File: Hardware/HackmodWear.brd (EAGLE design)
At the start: 110 parts, among them IC1 MSGEQ7N, Q2 2.5A/30V, U1 ATSAMD21G-A, U2 3.3V, U3 74AHC1G125, U4 DRV2605L, U5 OPA344, U6 ADMP401, U7 APDS-9960, Y1 32.768kHz

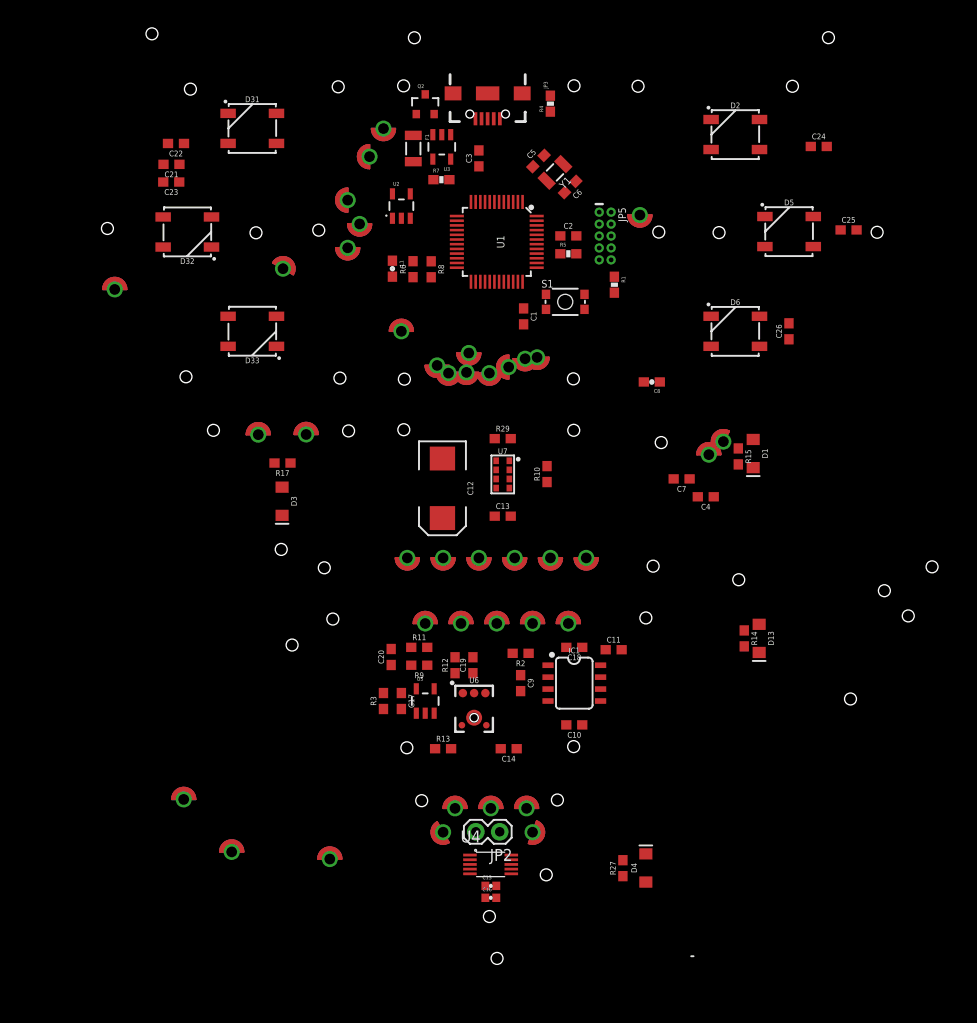
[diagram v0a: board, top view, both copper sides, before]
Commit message: Adding BOM and gerbers
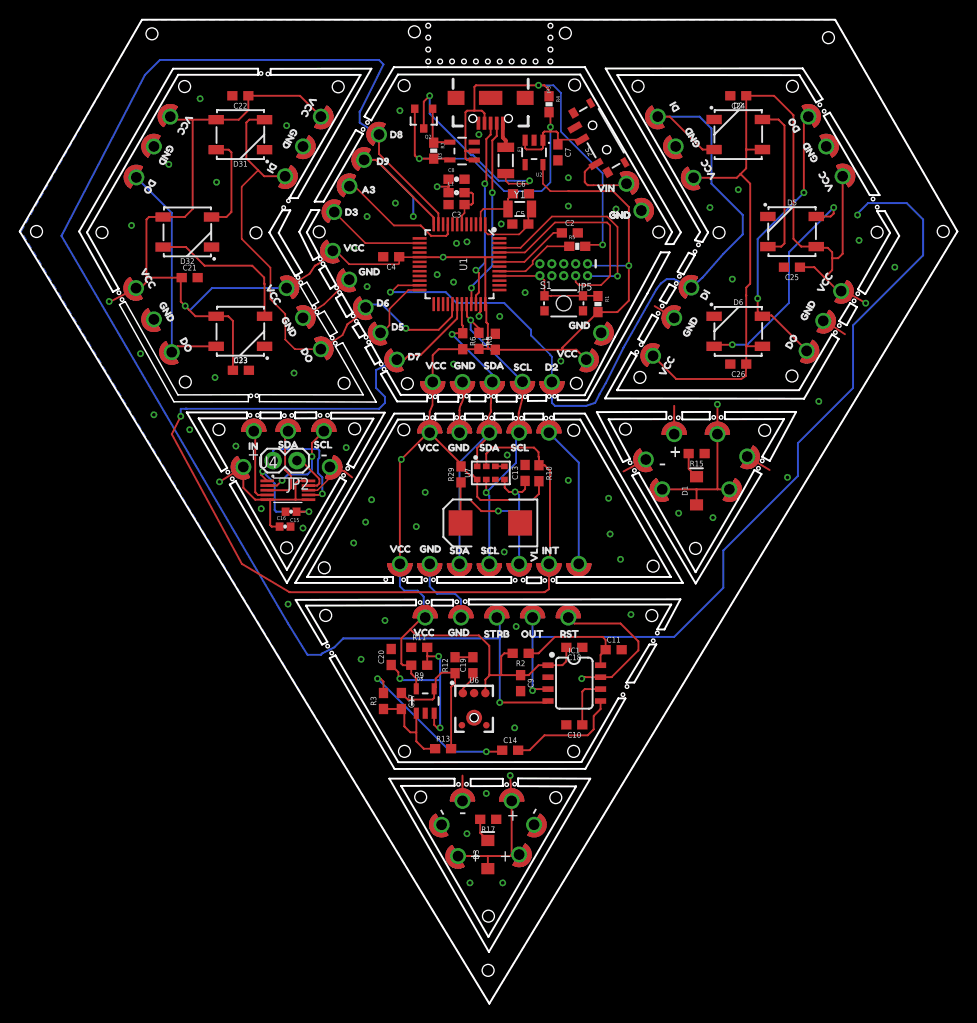
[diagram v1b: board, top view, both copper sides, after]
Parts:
- removed D13, D4: (no value), SparkFun-LED:LED-1206
- removed R14, R27: 330, SparkFun-Resistors:0603
- added J41, J42, J43, J44, J45, J46, J47, J48, J49, J50, J51, J52, J53, J54, J55, J56, J57, J58, J59, J60, J61, J62, J63, J64, J65, J66, J67, J68, J69, J70, J71, J72, J73, J74, J75, J76: (no value), SparkFun-Connectors:1X01
- added S2: (no value), SparkFun-Switches:SWITCH_SPST_SMD_A
- added U$1, U$10, U$12, U$19, U$21, U$26, U$29, U$37, U$38, U$40, U$42, U$45, U$49, U$50, U$55, U$56: (no value), buzzard_labels(2):GND2
- added U$11, U$51, U$57: (no value), buzzard_labels(2):DI6
- added U$13, U$23, U$24, U$60: (no value), buzzard_labels(2):SCL5
- added U$14, U$22, U$25, U$59: (no value), buzzard_labels(2):SDA4
- added U$15: (no value), buzzard_labels(2):STRB8
- added U$16, U$20, U$31, U$32, U$33, U$35, U$39, U$41, U$44, U$47, U$48, U$54, U$58: (no value), buzzard_labels(2):VCC1
- added U$17: (no value), buzzard_labels(2):RST9
- added U$18: (no value), buzzard_labels(2):OUT10
- added U$2: (no value), buzzard_labels(2):A313
- added U$27: (no value), buzzard_labels(2):INT23
- added U$28: (no value), buzzard_labels(2):VL22
- added U$3: (no value), buzzard_labels(2):D517
- added U$30: (no value), buzzard_labels(2):VCC21
- added U$34: (no value), buzzard_labels(2):D219
- added U$36: (no value), buzzard_labels(2):VIN20
- added U$4: (no value), buzzard_labels(2):D314
- added U$43, U$46, U$5, U$52, U$53: (no value), buzzard_labels(2):DO7
- added U$6: (no value), buzzard_labels(2):D616
- added U$62: (no value), buzzard_labels(2):IN3
- added U$7: (no value), buzzard_labels(2):D718
- added U$8: (no value), buzzard_labels(2):D811
- added U$9: (no value), buzzard_labels(2):D912
- moved J27 69.6 mm to (14.9, 92.1), turned to 60 degrees
- moved J38 58.9 mm to (54.2, 67.0), turned to 180 degrees
- moved J25 55.1 mm to (32.7, 95.2), turned to 240 degrees
- moved J12 53.7 mm to (51.0, 67.0), turned to 180 degrees
- moved J2 45.6 mm to (29.2, 61.8)
- moved J4 45.6 mm to (33.0, 61.8)
- moved J22 45.5 mm to (25.6, 61.8)
- moved U4 45.3 mm to (28.9, 55.4)
- moved C16 45.2 mm to (28.9, 51.6)
- moved C15 45.2 mm to (29.5, 53.2), turned to 180 degrees
- moved JP2 45.0 mm to (30.2, 58.6)
- moved J20 44.5 mm to (33.7, 57.9)
- moved J1 44.3 mm to (24.4, 57.9)
- moved R17 43.8 mm to (50.5, 20.4)
- moved D3 43.5 mm to (50.5, 16.7), turned to 90 degrees
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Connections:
- removed net DI1: J26.P$1, J32.P$1
- removed net INT: J40.P$1, R10.1, U7.2
- removed net VL: C12.A, C13.1, J24.P$1, R29.1, U7.5
- net 3.3V: now also J17.P$1, J44.P$1, J45.P$1, J47.P$1, J52.P$1, J56.P$1, J57.P$1, J60.P$1, J62.P$1, J64.P$1, J66.P$1, J68.P$1, J70.P$1, J73.P$1, J76.P$1; no longer D13.A, D4.A
- net A0: no longer IC1.3, J37.P$1, J5.P$1
- net A1: no longer J10.P$1
- net A2: no longer J11.P$1
- net A3: now also IC1.3, J10.P$1, J37.P$1; no longer J3.P$1
- net D0/RXI: no longer J21.P$1
- net D1/TXO: no longer J19.P$1
- net D10/SS: no longer J17.P$1
- net D11/MOSI: no longer J14.P$1
- net D12/MISO: no longer J16.P$1
- net D13/SCK: no longer J15.P$1
- net D2: now also D2.4, J14.P$1, J42.P$1, J53.P$1
- net D5: now also C12.A, C13.1, J24.P$1, J3.P$1, R29.1, U7.5
- net D6: now also J26.P$1, J32.P$1
- net D7: now also J40.P$1, J5.P$1, R10.1, U7.2
- net DO: now also J41.P$1, J54.P$1; no longer D2.4
- net DOUT: now also J48.P$1, J50.P$1
- net GND: now also J11.P$1, J19.P$1, J43.P$1, J46.P$1, J49.P$1, J51.P$1, J55.P$1, J58.P$1, J59.P$1, J61.P$1, J63.P$1, J65.P$1, J67.P$1, J69.P$1, J72.P$1, J75.P$1; no longer R14.1, R27.1
- net N$21: now also J71.P$1, S2.3; no longer D4.C, R27.2
- net N$8: now also J21.P$1, J74.P$1; no longer D13.C, R14.2
- net SCL: now also J15.P$1
- net SDA: now also J16.P$1
- net VIN: now also S2.2
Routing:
- net 3.3V: track 0.00 -> 417.0 mm, vias 0 -> 10
- net D9: track 0.00 -> 163.5 mm, vias 0 -> 2
- net A3: track 0.00 -> 160.5 mm, vias 0 -> 2
- net D8: track 0.00 -> 154.5 mm, vias 0 -> 1
- net D5: track 0.00 -> 141.2 mm, vias 0 -> 3
- net D7: track 0.00 -> 113.3 mm, vias 0 -> 1
- net D2: track 0.00 -> 86.3 mm, vias 0 -> 1
- net SCL: track 0.00 -> 74.0 mm, vias 0 -> 4
- net SDA: track 0.00 -> 72.3 mm, vias 0 -> 1
- net D6: track 0.00 -> 54.9 mm, vias 0 -> 1
- net D3: track 0.00 -> 52.4 mm
- net GND: track 0.00 -> 45.2 mm, vias 0 -> 62
- net ID: track 0.00 -> 44.5 mm, vias 0 -> 2
- net VIN: track 0.00 -> 42.9 mm, vias 0 -> 2
- net DOUT: track 0.00 -> 30.1 mm, vias 0 -> 2
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- added copper zone on layer 15, net 3.3V
- added copper zone on layer 1, net GND
- added copper zone on layer 16, net GND
- added copper zone on layer 2, net GND
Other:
- board outline added: 99.9 x 104.8 mm
- board text added: "+"
- board text added: "-"
